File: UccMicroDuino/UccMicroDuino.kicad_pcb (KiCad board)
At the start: 2 copper layers, 51.4 x 48.3 mm, 14 parts, among them J1 USB_PCB_A, J2 Header, U1 ATtiny85-20S

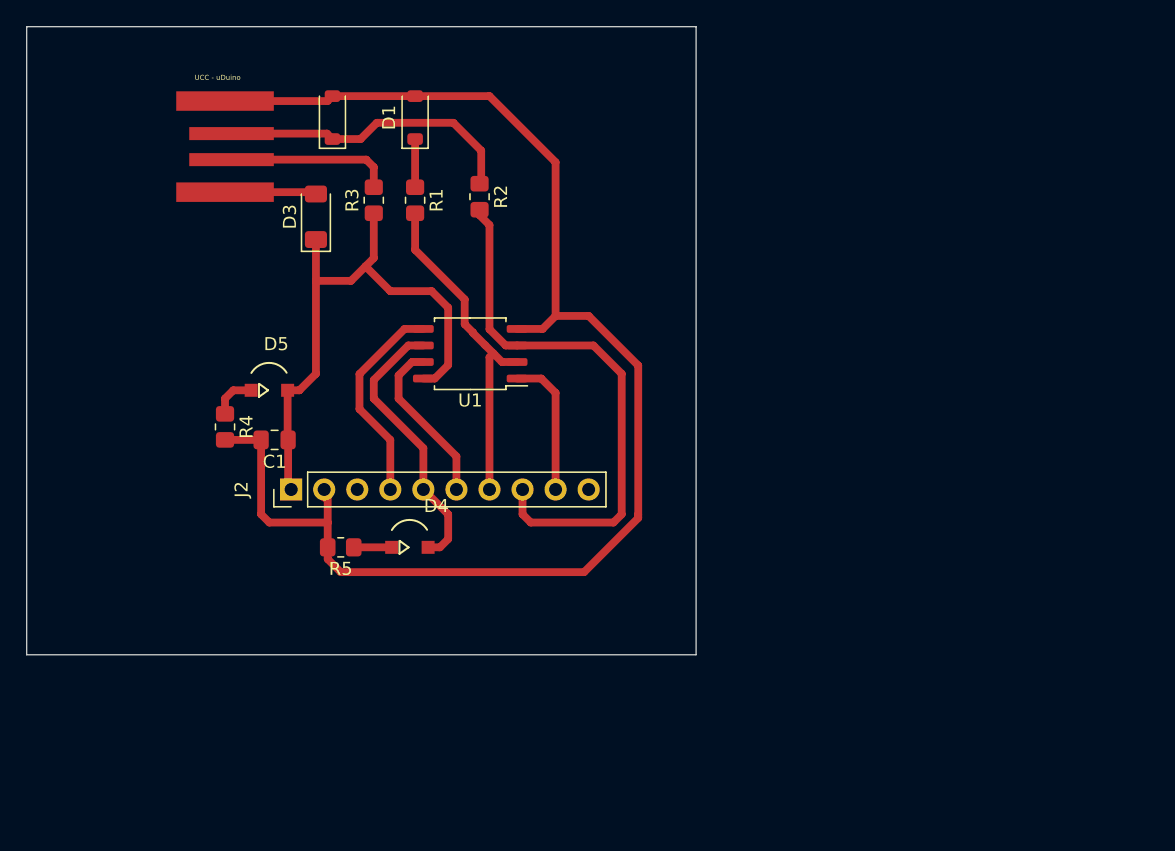
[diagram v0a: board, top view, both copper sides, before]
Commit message: Arreglando la placa
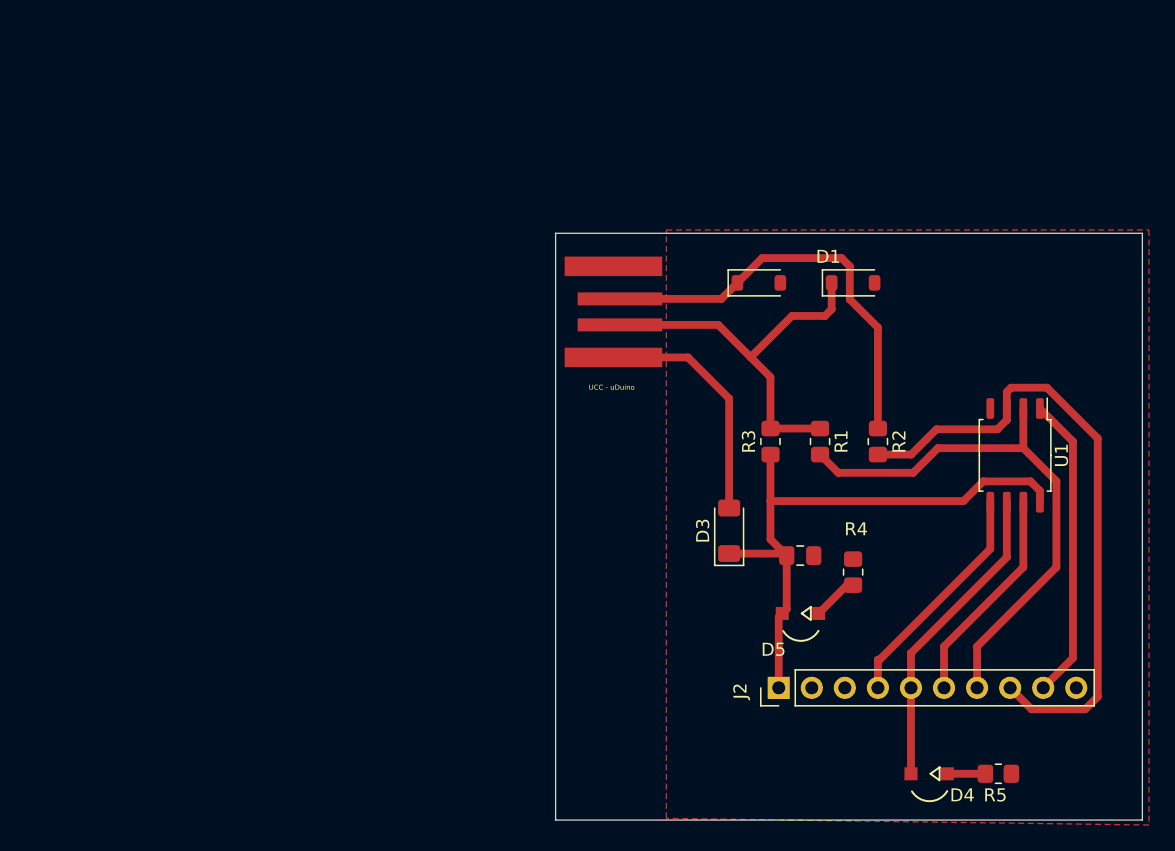
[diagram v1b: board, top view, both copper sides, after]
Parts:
- moved R5 53.4 mm to (169.3, 96.1), turned to 0 degrees
- moved R4 49.5 mm to (158.1, 80.6), turned to 90 degrees
- moved D5 43.5 mm to (153.7, 83.8), turned to 180 degrees
- moved D4 42.8 mm to (163.6, 96.1), turned to 180 degrees
- moved U1 42.6 mm to (170.6, 71.7), turned to -90 degrees
- moved C1 41.4 mm to (154.1, 79.4), turned to 0 degrees
- moved J2 40.4 mm to (152.4, 89.5)
- moved D3 39.9 mm to (148.6, 77.5)
- moved R1 36.2 mm to (155.6, 70.6)
- moved D1 36.0 mm to (158.1, 58.4), turned to 0 degrees
- moved R2 35.9 mm to (160.0, 70.6)
- moved R3 35.7 mm to (151.8, 70.6)
- moved D2 35.1 mm to (150.9, 58.4), turned to 0 degrees
- moved J1 32.4 mm to (139.9, 60.6)
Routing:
- net GND: track 108.5 -> 0.00 mm
- net Net-(J2-Pin_7): track 25.9 -> 42.0 mm
- net Net-(D1-K): track 16.4 -> 30.8 mm
- net Net-(J2-Pin_9): track 10.8 -> 23.5 mm
- net Net-(D3-A): track 7.04 -> 18.6 mm
- net Net-(D2-K): track 23.4 -> 32.6 mm
- net Net-(J2-Pin_8): track 41.9 -> 49.6 mm
- net Net-(J2-Pin_6): track 12.9 -> 16.8 mm
- net Net-(D4-A): track 21.3 -> 23.9 mm
- net +5V: track 43.5 -> 45.7 mm
- net Net-(J2-Pin_4): track 16.2 -> 17.9 mm
- added copper zone on F.Cu, net GND
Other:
- board size 51.4 x 48.3 mm -> 45.1 x 45.1 mm
